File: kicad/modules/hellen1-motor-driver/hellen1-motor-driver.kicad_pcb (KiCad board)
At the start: 4 copper layers, 13.8 x 10 mm, 17 parts, among them M821 Module-motor-driver-0.1, U821 TLE9201SG

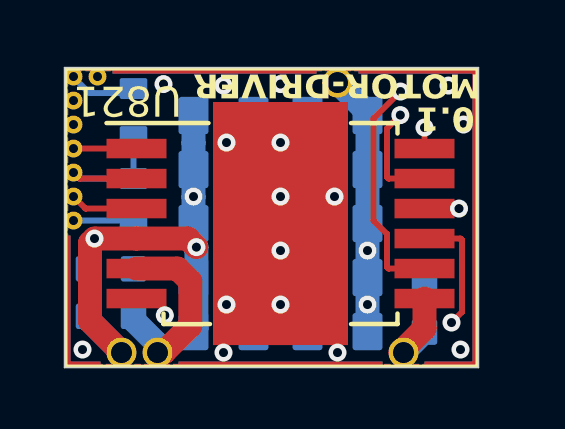
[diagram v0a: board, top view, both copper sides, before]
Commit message: #376 motor-driver
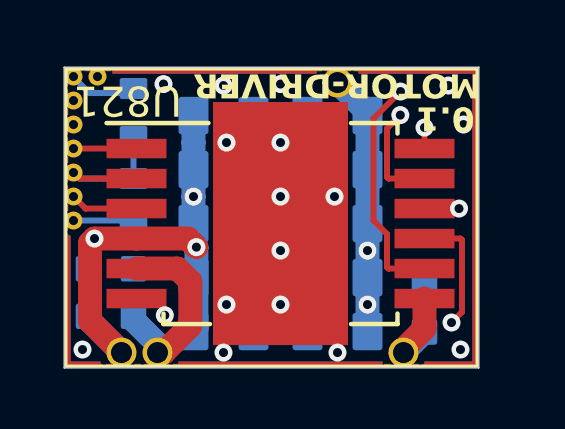
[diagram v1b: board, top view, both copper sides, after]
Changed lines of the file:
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@@
     )
     (pad_to_mask_clearance 0)
-    (aux_axis_origin 84.4 78)
-    (grid_origin 84.4 78)
+    (aux_axis_origin 84.39 78.01)
+    (grid_origin 84.39 78.01)
     (pcbplotparams
       (layerselection 0x00410fc_ffffffff)
@@
     )
   )
-  (gr_rect (start 84.4 68) (end 98.2 78)
+  (gr_rect (start 84.39 67.99) (end 98.21 78.01)
     (stroke (width 0.05) (type default)) (fill none) (layer "Edge.Cuts"))
-  (gr_rect (start 84.4 68) (end 98.2 78)
+  (gr_rect (start 84.39 67.99) (end 98.21 78.01)
     (stroke (width 0.1) (type default)) (fill none) (layer "User.1"))
   (gr_text "0.1" (at 96.2 69.2 -90) (layer "B.SilkS")
